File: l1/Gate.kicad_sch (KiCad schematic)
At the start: 14 parts, among them J203 Conn_01x04, SW202 IMU RST, U204 STM32F103Cx, Y202 8Mhz

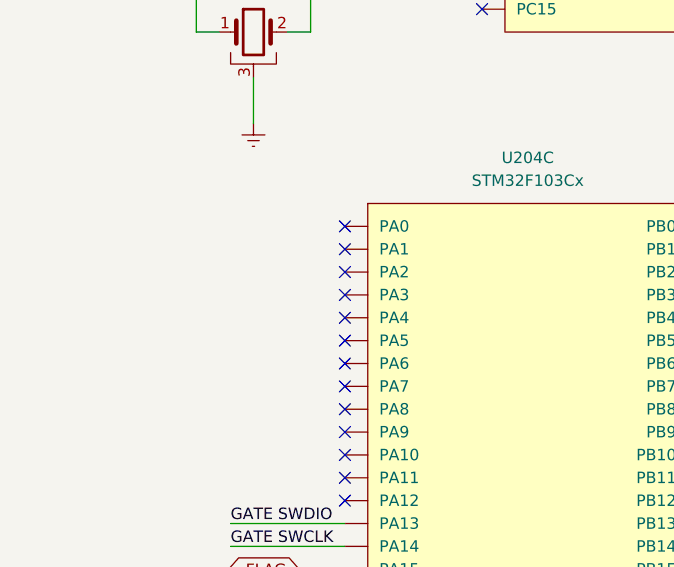
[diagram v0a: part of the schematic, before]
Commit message: l1
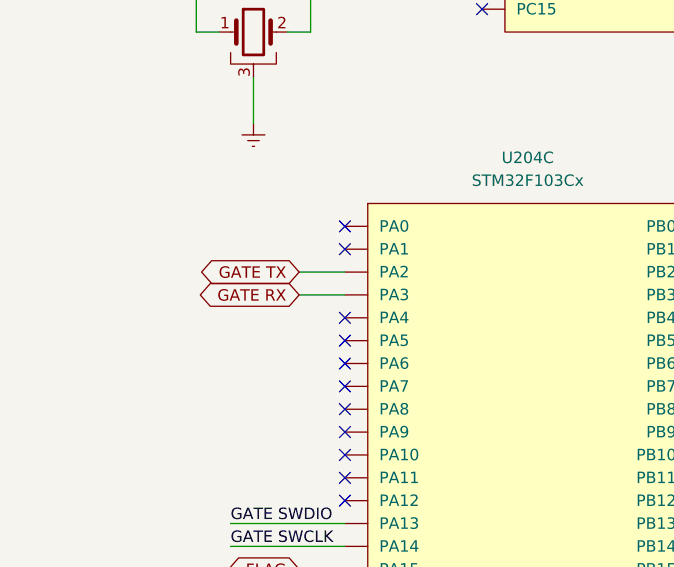
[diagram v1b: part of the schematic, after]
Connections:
- net GATE TX: now reaches U204.12 (PA2)
- net GATE RX: now reaches U204.13 (PA3)
- no-connect marks 31 -> 29
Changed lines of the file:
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@@
-	)
-	(no_connect
-		(at 68.58 128.27)
 	)
 	(no_connect
@@
 		(at 109.22 125.73)
 	)
-	(no_connect
-		(at 68.58 130.81)
-	)
 	(wire
 		(pts
@@
 	(wire
 		(pts
+			(xy 63.5 130.81) (xy 68.58 130.81)
+		)
+		(stroke
+			(width 0)
+			(type default)
+		)
+	)
+	(wire
+		(pts
 			(xy 86.36 182.88) (xy 73.66 182.88)
 		)
@@
 		(pts
 			(xy 83.82 88.9) (xy 64.77 88.9)
+		)
+		(stroke
+			(width 0)
+			(type default)
+		)
+	)
+	(wire
+		(pts
+			(xy 63.5 128.27) (xy 68.58 128.27)
 		)
 		(stroke
@@
 			(effects
 				(font
+					(size 1.27 1.27)
+				)
+				(justify right)
+				(hide yes)
+			)
+		)
+	)
+	(global_label "GATE TX"
+		(shape bidirectional)
+		(at 63.5 128.27 180)
+		(fields_autoplaced yes)
+		(effects
+			(font
+				(size 1.27 1.27)
+			)
+			(justify right)
+		)
+		(property "Intersheetrefs" "${INTERSHEET_REFS}"
+			(at 51.7836 128.27 0)
+			(effects
+				(font
+					(size 1.27 1.27)
+				)
+				(justify right)
+				(hide yes)
+			)
+		)
+	)
+	(global_label "GATE RX"
+		(shape bidirectional)
+		(at 63.5 130.81 180)
+		(fields_autoplaced yes)
+		(effects
+			(font
+				(size 1.27 1.27)
+			)
+			(justify right)
+		)
+		(property "Intersheetrefs" "${INTERSHEET_REFS}"
+			(at 51.4812 130.81 0)
+			(effects
+				(font

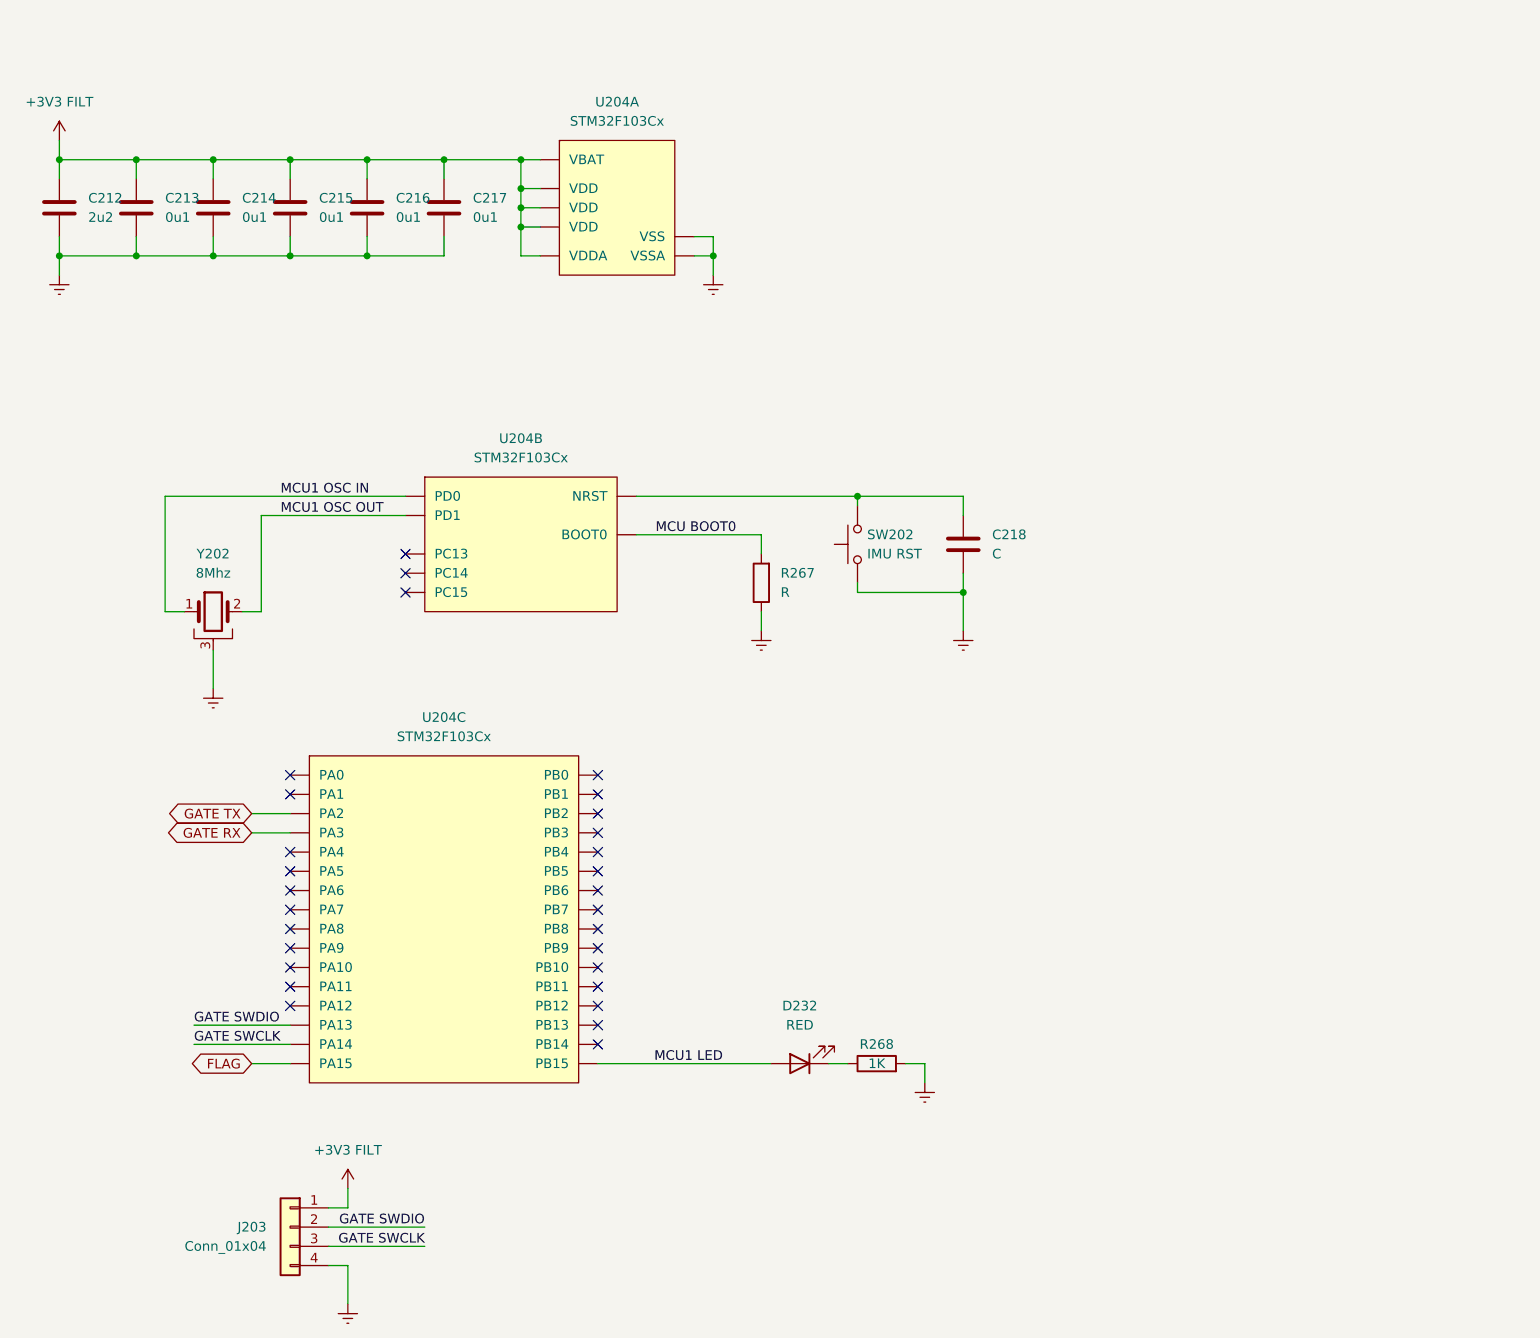
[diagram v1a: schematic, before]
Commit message: breakout
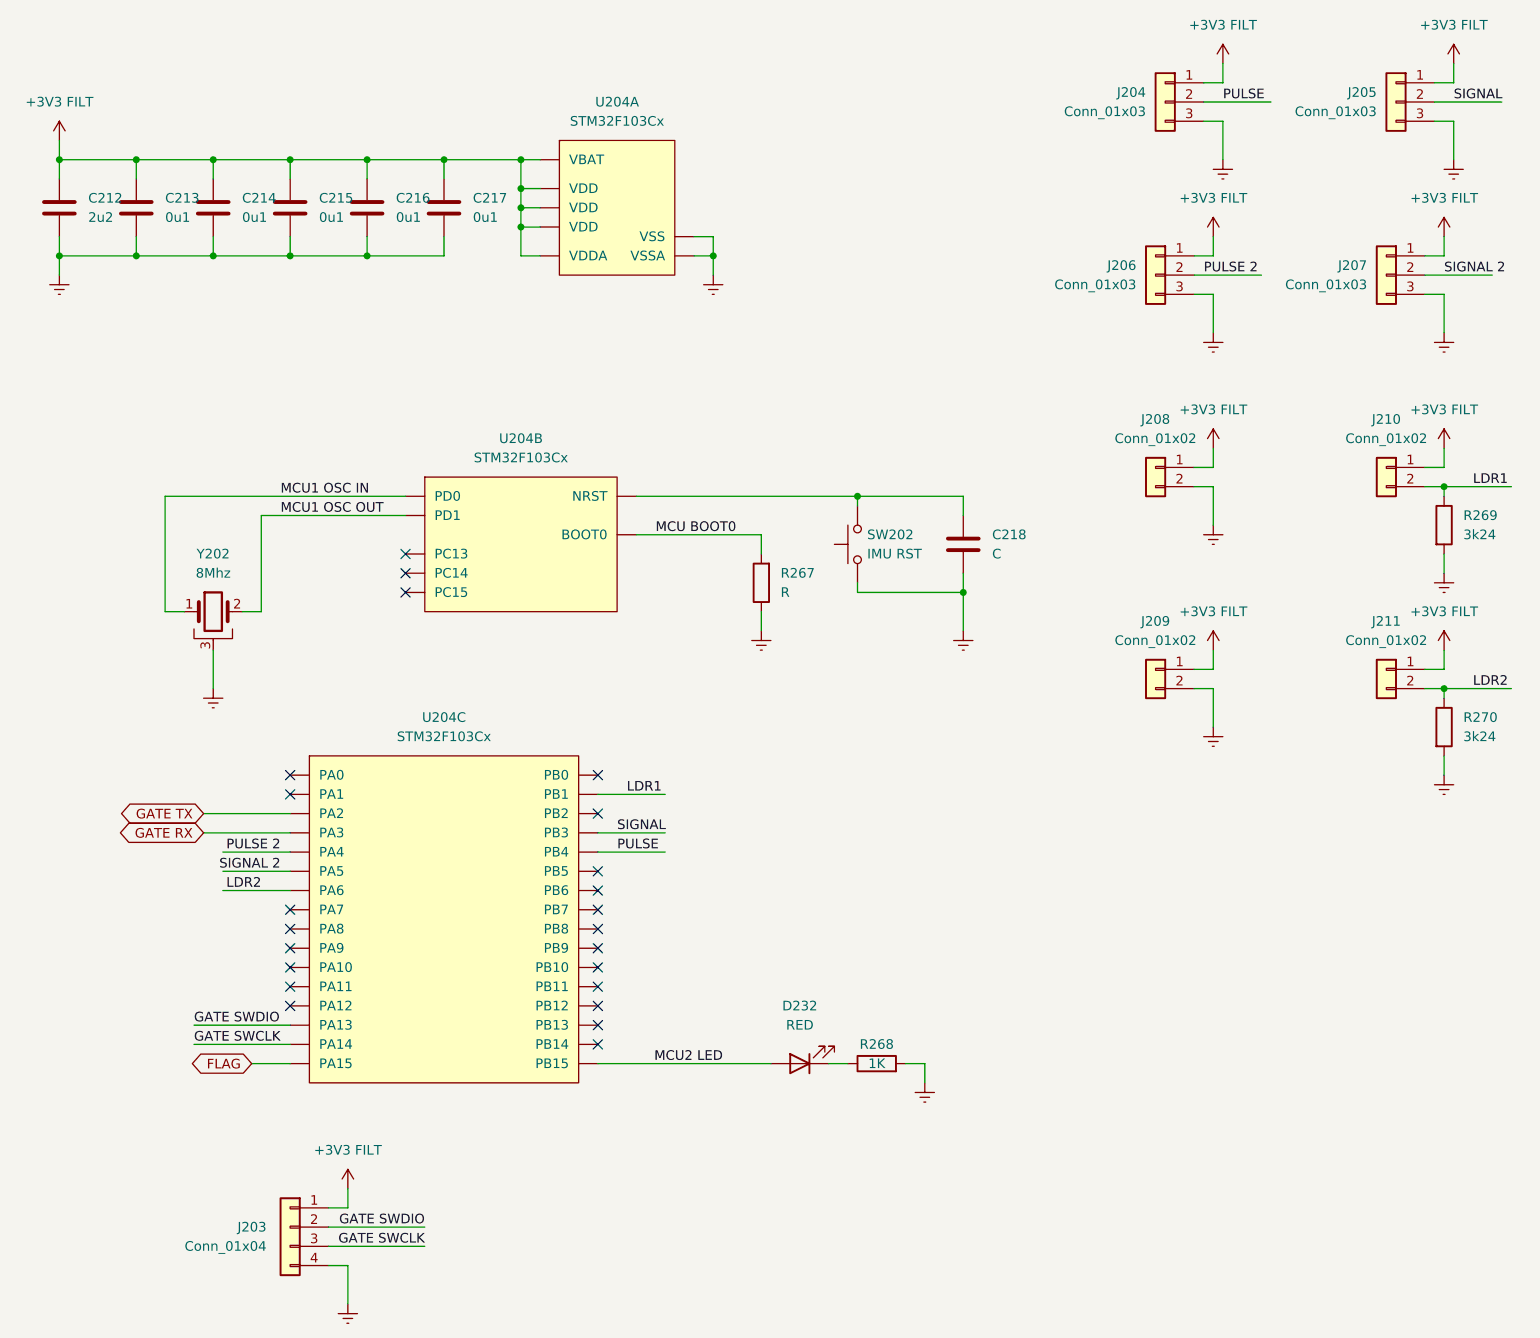
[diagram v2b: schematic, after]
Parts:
- added J204, J205, J206, J207: Conn_01x03, Connector_PinHeader_2.54mm:PinHeader_1x03_P2.54mm_Vertical, symbol Connector_Generic:Conn_01x03
- added J208, J209, J210, J211: Conn_01x02, Connector_PinHeader_2.54mm:PinHeader_1x02_P2.54mm_Vertical, symbol Connector_Generic:Conn_01x02
- added R269, R270: 3k24, Library:res0603, symbol Device:R
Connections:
- net +3V3 FILT: now also J204.1 (Pin_1), J205.1 (Pin_1), J206.1 (Pin_1), J207.1 (Pin_1), J208.1 (Pin_1), J209.1 (Pin_1), J210.1 (Pin_1), J211.1 (Pin_1)
- net GNDREF: now also J204.3 (Pin_3), J205.3 (Pin_3), J206.3 (Pin_3), J207.3 (Pin_3), J208.2 (Pin_2), J209.2 (Pin_2), R269.2, R270.2
- net PULSE 2: now reaches U204.14 (PA4)
- net PULSE 2: now also J206.2 (Pin_2)
- net SIGNAL 2: now reaches U204.15 (PA5)
- net SIGNAL 2: now also J207.2 (Pin_2)
- net LDR2: now reaches U204.16 (PA6)
- net LDR2: now also J211.2 (Pin_2), R270.1
- net LDR1: now reaches U204.19 (PB1)
- net LDR1: now also J210.2 (Pin_2), R269.1
- net SIGNAL: now reaches U204.39 (PB3)
- net SIGNAL: now also J205.2 (Pin_2)
- net PULSE: now reaches U204.40 (PB4)
- net PULSE: now also J204.2 (Pin_2)
- net MCU1 LED renamed MCU2 LED
- no-connect marks 29 -> 23
